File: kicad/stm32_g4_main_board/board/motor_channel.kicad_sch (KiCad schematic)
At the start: 14 parts, among them J1 MR30PW-M, U1 DRV8304HRHAR

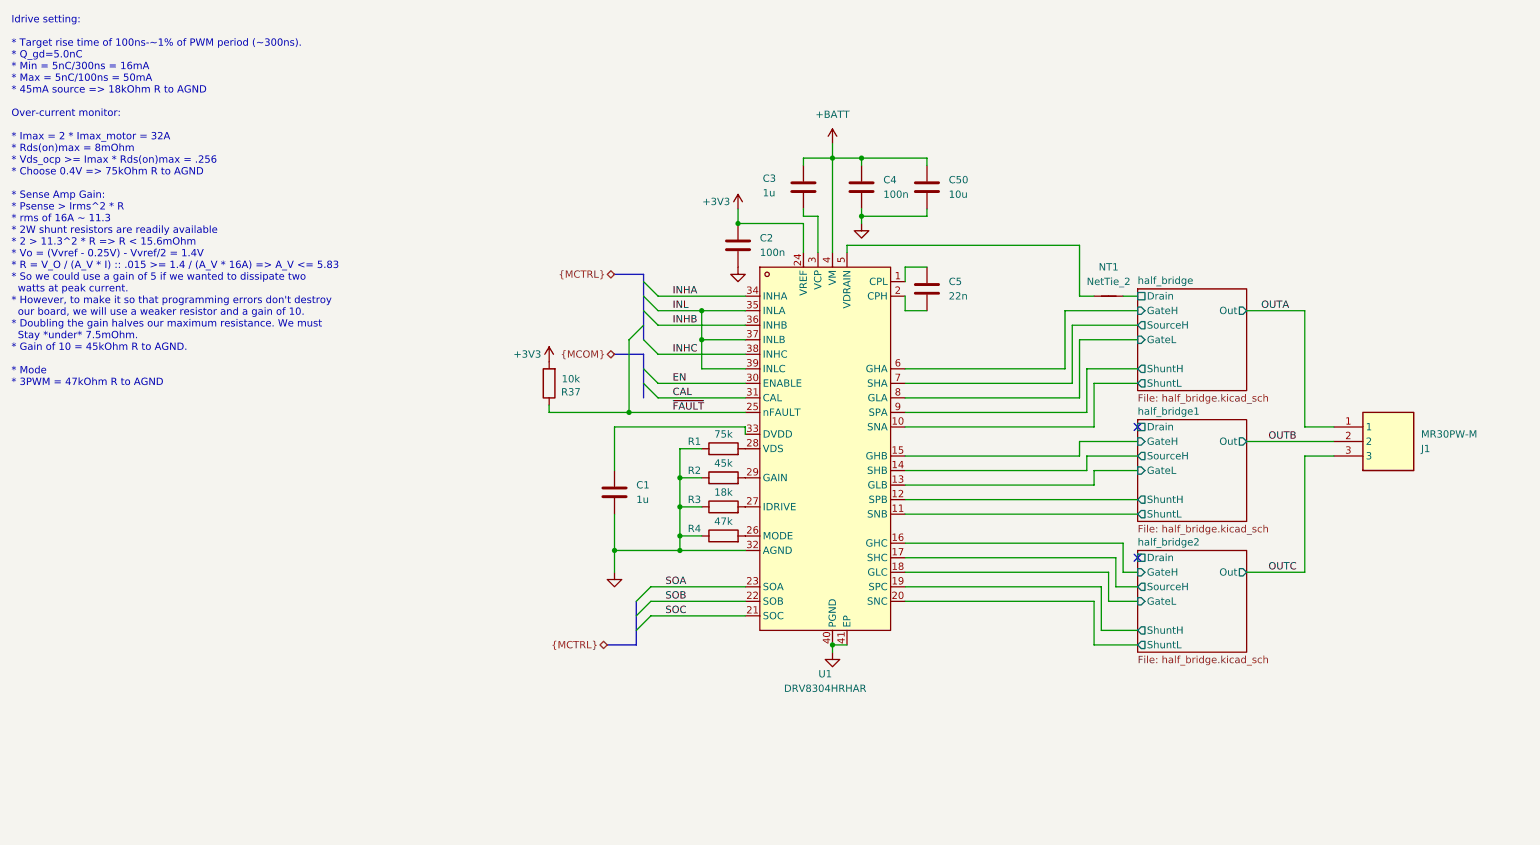
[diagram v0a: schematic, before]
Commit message: WIP - v2 board
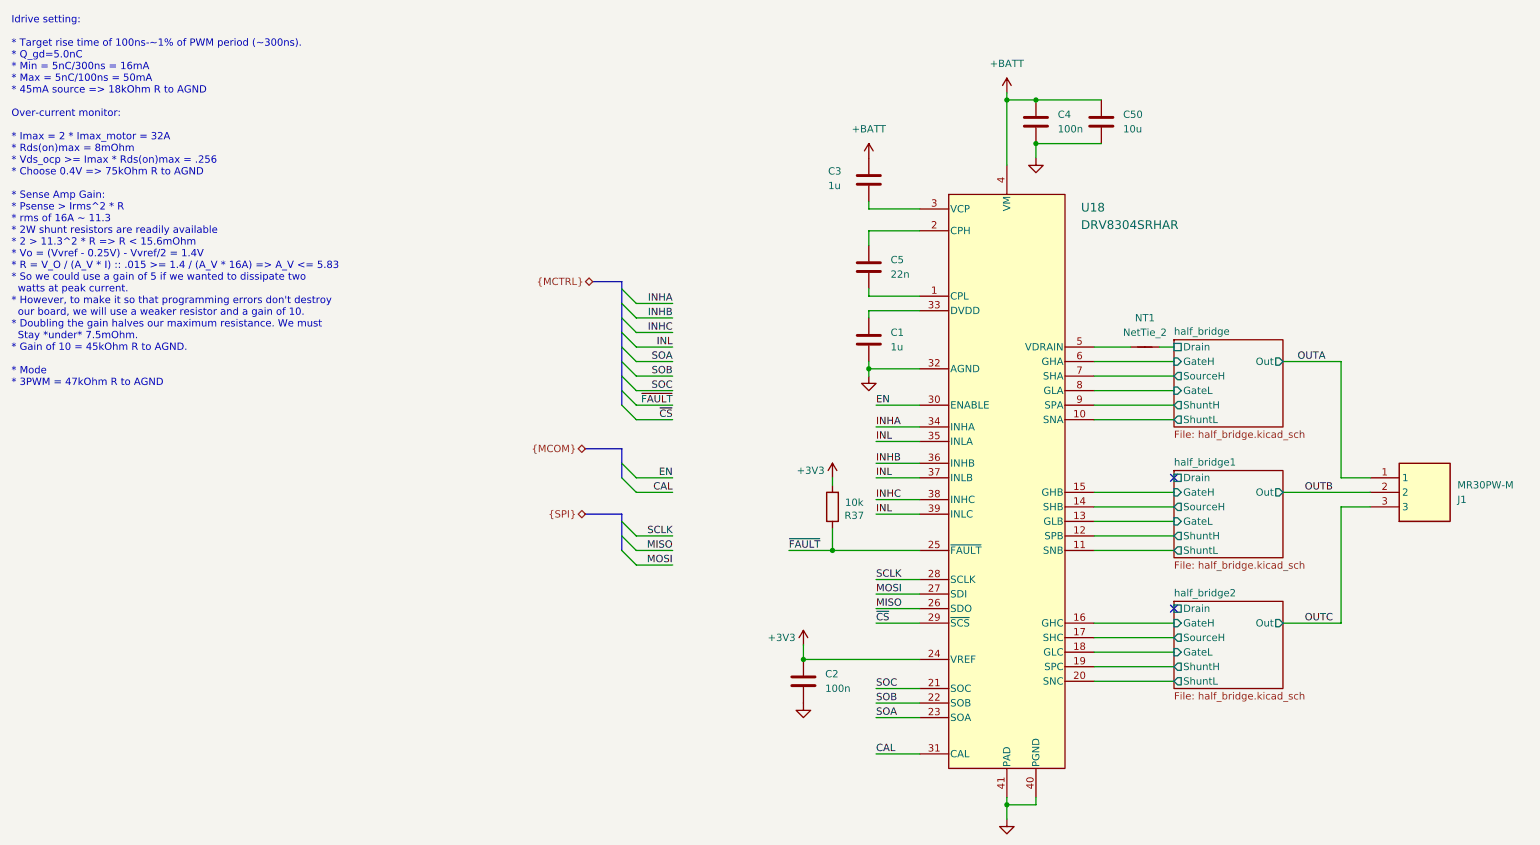
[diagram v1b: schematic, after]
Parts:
- removed R1: 75k, Resistor_SMD:R_0805_2012Metric, symbol Device:R
- removed R2: 45k, Resistor_SMD:R_0805_2012Metric, symbol Device:R
- removed R3: 18k, Resistor_SMD:R_0805_2012Metric, symbol Device:R
- removed R4: 47k, Resistor_SMD:R_0805_2012Metric, symbol Device:R
- removed U1: DRV8304HRHAR, jaguilar:C2677109_VQFN-40_L6_0-W6_0-P0_50-TL-EP, symbol EasyEDA:DRV8304HRHAR
- added U18: DRV8304SRHAR, jaguilar:QFN-40_EP_6.15x6.15_Pitch0.5mm, symbol jaguilar:DRV8304SRHAR
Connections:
- net +3V3: now also U18.24 (VREF)
- net +BATT: now also U18.4 (VM)
- net CAL: now also U18.31 (CAL)
- net EN: now also U18.30 (ENABLE)
- net GND: now also U18.32 (AGND), U18.40 (PGND), U18.41 (PAD)
- net INHA: now also U18.34 (INHA)
- net INHB: now also U18.36 (INHB)
- net INHC: now also U18.38 (INHC)
- net INL: now also U18.35 (INLA), U18.37 (INLB), U18.39 (INLC)
- net SOA: now also U18.23 (SOA)
- net SOB: now also U18.22 (SOB)
- net SOC: now also U18.21 (SOC)
- net half_bridge/GateH: now also U18.6 (GHA)
- net half_bridge/GateL: now also U18.8 (GLA)
- net half_bridge/ShuntH: now also U18.9 (SPA)
- net half_bridge/ShuntL: now also U18.10 (SNA)
- net half_bridge/SourceH: now also U18.7 (SHA)
- net half_bridge1/GateH: now also U18.15 (GHB)
- net half_bridge1/GateL: now also U18.13 (GLB)
- net half_bridge1/ShuntH: now also U18.12 (SPB)
- net half_bridge1/ShuntL: now also U18.11 (SNB)
- net half_bridge1/SourceH: now also U18.14 (SHB)
- net half_bridge2/GateH: now also U18.16 (GHC)
- net half_bridge2/GateL: now also U18.18 (GLC)
- net half_bridge2/ShuntH: now also U18.19 (SPC)
- net half_bridge2/ShuntL: now also U18.20 (SNC)
- net half_bridge2/SourceH: now also U18.17 (SHC)
- net ~{FAULT}: now also U18.25 (~{FAULT})
- net at C5.1: now also U18.2 (CPH)
- net at C5.2: now also U18.1 (CPL)
- net at C3.2: now also U18.3 (VCP)
- net at C1.1: now also U18.33 (DVDD)
- net at NT1.1: now also U18.5 (VDRAIN)
- new net MISO: U18.26 (SDO)
- new net MOSI: U18.27 (SDI)
- new net SCLK: U18.28 (SCLK)
- new net ~{CS}: U18.29 (~{SCS})
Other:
- moved on the sheet: C1, C2, C3, C4, C5, C50, J1, NT1, R37
